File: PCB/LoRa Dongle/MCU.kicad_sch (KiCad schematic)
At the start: 25 parts, among them U3 AP2112K-3.3, U4 STM32WLE5CCUx, Y1 Crystal_GND24

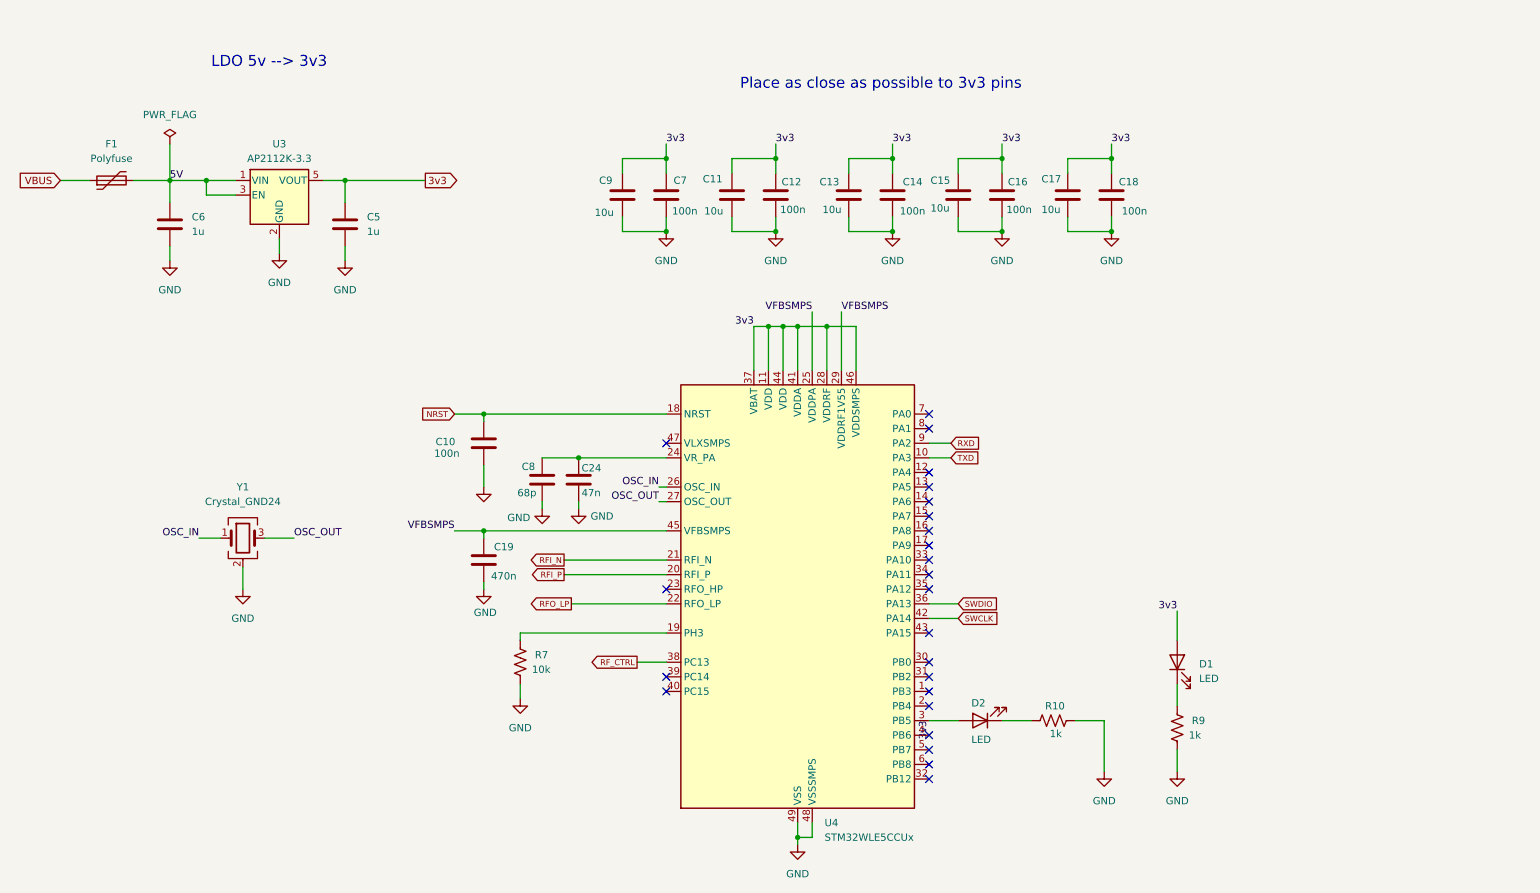
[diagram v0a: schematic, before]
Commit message: first layout
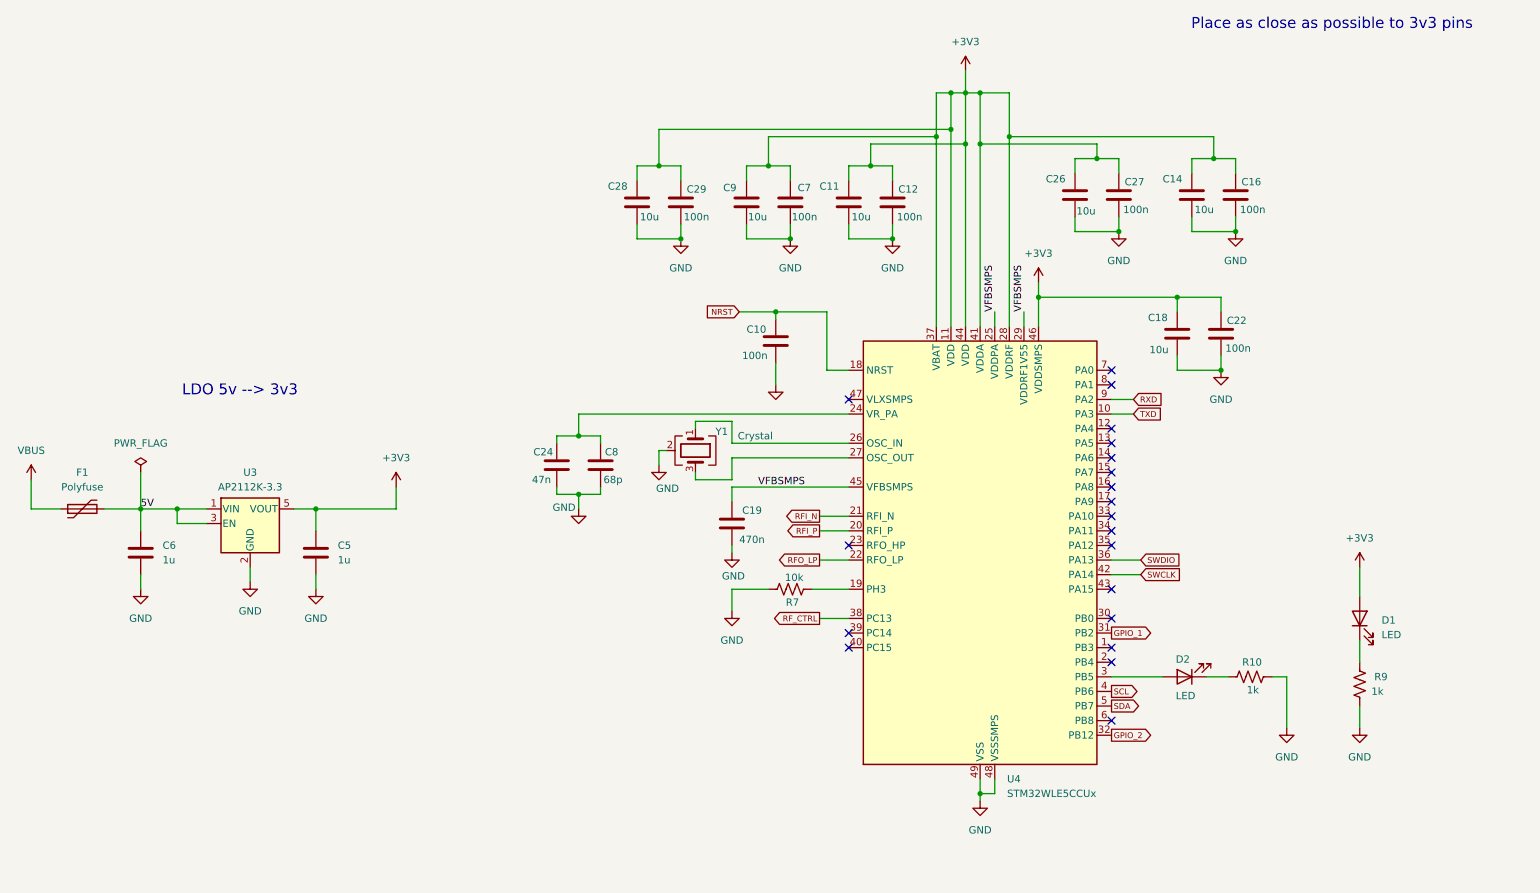
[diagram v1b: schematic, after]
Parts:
- removed C13, C15, C17: 10u, PCM_JLCPCB:C_0603, symbol Device:C
- added C22, C27, C29: 100n, PCM_JLCPCB:C_0402, symbol Device:C
- added C26, C28: 10u, PCM_JLCPCB:C_0402, symbol Device:C
- C10, C11, C12, C16, C19, C24, C5, C6, C7, C8, C9: footprint PCM_JLCPCB:C_0603 -> PCM_JLCPCB:C_0402
- C14, C18: value 100n -> 10u; footprint PCM_JLCPCB:C_0603 -> PCM_JLCPCB:C_0402
- F1: footprint Fuse:Fuse_1812_4532Metric -> Fuse:Fuse_1210_3225Metric
- R10, R7, R9: footprint PCM_JLCPCB:R_0603 -> PCM_JLCPCB:R_0402
- Y1: value Crystal_GND24 -> Crystal
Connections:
- net GND: now also R7.1, C22.2, C26.2, C27.2, C28.2, C29.2; no longer R7.2
- net at U4.19 (PH3): now also R7.2; no longer R7.1
- net GPIO_1: now reaches U4.31 (PB2)
- net GPIO_2: now reaches U4.32 (PB12)
- net SCL: now reaches U4.4 (PB6)
- net SDA: now reaches U4.5 (PB7)
- net 3v3 renamed +3V3
- net +3V3: now also C22.1, C26.1, C27.1, C28.1, C29.1; no longer D2.2 (A), U4.3 (PB5)
- net OSC_IN: no longer names the net of U4.26 (OSC_IN), Y1.1
- net OSC_OUT: no longer names the net of U4.27 (OSC_OUT), Y1.3
- new net: D2.2 (A), U4.3 (PB5)
- no-connect marks 24 -> 20
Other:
- moved on the sheet: C19, C5, C6, D1, D2, F1, R10, R7, R9, U3, U4, Y1
